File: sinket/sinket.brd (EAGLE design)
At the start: 36 x 36 mm, 25 parts, among them IC1 ATTINY85-20PU, IC2 TS2940CP50S

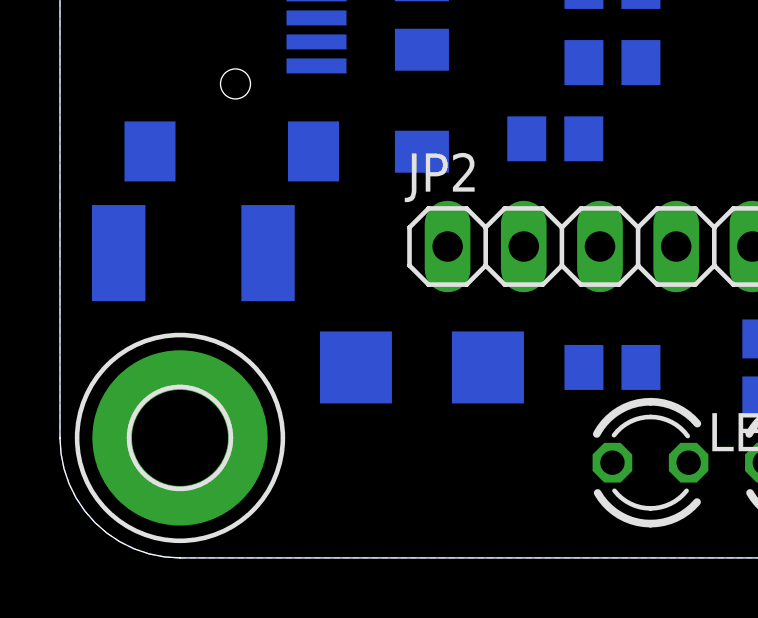
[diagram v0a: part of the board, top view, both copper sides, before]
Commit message: change fuse package
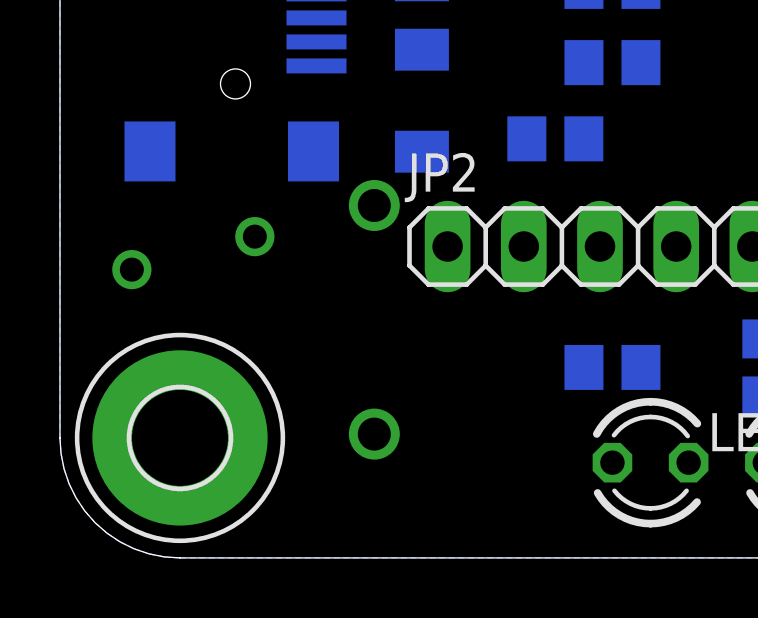
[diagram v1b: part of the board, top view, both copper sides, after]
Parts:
- D3: value MBRS240LT3 -> 1N5817-B; device diode:SMB -> diode:DO41-7.6
- F1: value SIBA_194600 -> (none); device n39:PTC-FUSE-1812 -> n39:LP60-050
- moved D3 2.25 mm to (10.5, 7.94), turned to 270 degrees
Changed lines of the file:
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@@
 <setting verticaltext="up"/>
 </settings>
-<grid distance="25" unitdist="mil" unit="mil" style="dots" multiple="1" display="yes" altdistance="25" altunitdist="mil" altunit="mil"/>
+<grid distance="12.5" unitdist="mil" unit="mil" style="dots" multiple="1" display="yes" altdistance="25" altunitdist="mil" altunit="mil"/>
 <layers>
 <layer number="1" name="Top" color="4" fill="1" visible="yes" active="yes"/>
@@
 <element name="LED2" library="led" package="LED3MM" value="green" x="24.765" y="3.175"/>
 <element name="C1" library="rcl" package="C0805" value="100n" x="29.845" y="14.605" rot="MR0"/>
-<element name="D3" library="diode" package="SMB" value="MBRS240LT3" x="12.065" y="6.35" rot="MR0"/>
+<element name="D3" library="diode" package="DO41-7.6" value="1N5817-B" x="10.4775" y="7.9375" rot="MR270"/>
 <element name="IC2" library="n39" package="TO-252" value="TS2940CP50S" x="19.685" y="31.75" rot="MR90">
 <attribute name="REICHELT" value="TS 2940 CP50" x="19.685" y="31.75" size="1.778" layer="28" rot="MR90" display="off"/>
@@
 <element name="C2" library="rcl" package="C025-030X050" value="470n" x="7.62" y="26.035" rot="R180"/>
 <element name="C3" library="rcl" package="E2,5-6" value="47u" x="12.065" y="31.75" rot="R270"/>
-<element name="F1" library="n39" package="PTC-FUSE-1812" value="SIBA_194600" x="4.445" y="10.16" rot="MR180"/>
+<element name="F1" library="n39" package="LP60-050" value="" x="4.445" y="10.16" rot="MR180"/>
 </elements>
 <signals>
@@
 <wire x1="23.08" y1="10.38" x2="17.46" y2="13.97" width="0" layer="19" extent="16-16"/>
 <wire x1="23.495" y1="7.3" x2="23.08" y2="10.38" width="0" layer="19" extent="16-16"/>
-<wire x1="14.265" y1="6.35" x2="17.46" y2="13.97" width="0" layer="19" extent="16-16"/>
+<wire x1="10.4775" y1="11.7475" x2="17.46" y2="13.97" width="0" layer="19" extent="16-16"/>
 <wire x1="30.795" y1="14.605" x2="23.08" y2="10.38" width="0" layer="19" extent="16-16"/>
 <wire x1="33.655" y1="13.655" x2="30.795" y2="14.605" width="0" layer="19" extent="16-16"/>
@@
 <contactref element="F1" pad="P$1"/>
 <wire x1="12.92" y1="10.38" x2="8.55" y2="16.4" width="0" layer="19" extent="16-16"/>
-<wire x1="1.955" y1="10.16" x2="8.55" y2="16.4" width="0" layer="19" extent="16-16"/>
+<wire x1="2.395" y1="9.61" x2="8.55" y2="16.4" width="0" layer="19" extent="16-16"/>
 </signal>
 <signal name="GND" class="1">
@@
 <contactref element="F1" pad="P$2"/>
 <contactref element="D3" pad="A"/>
-<wire x1="9.865" y1="6.35" x2="6.935" y2="10.16" width="0" layer="19" extent="16-16"/>
+<wire x1="10.4775" y1="4.1275" x2="6.495" y2="10.71" width="0" layer="19" extent="16-16"/>
 </signal>
 </signals>
